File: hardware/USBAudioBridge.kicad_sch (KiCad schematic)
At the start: 0 parts

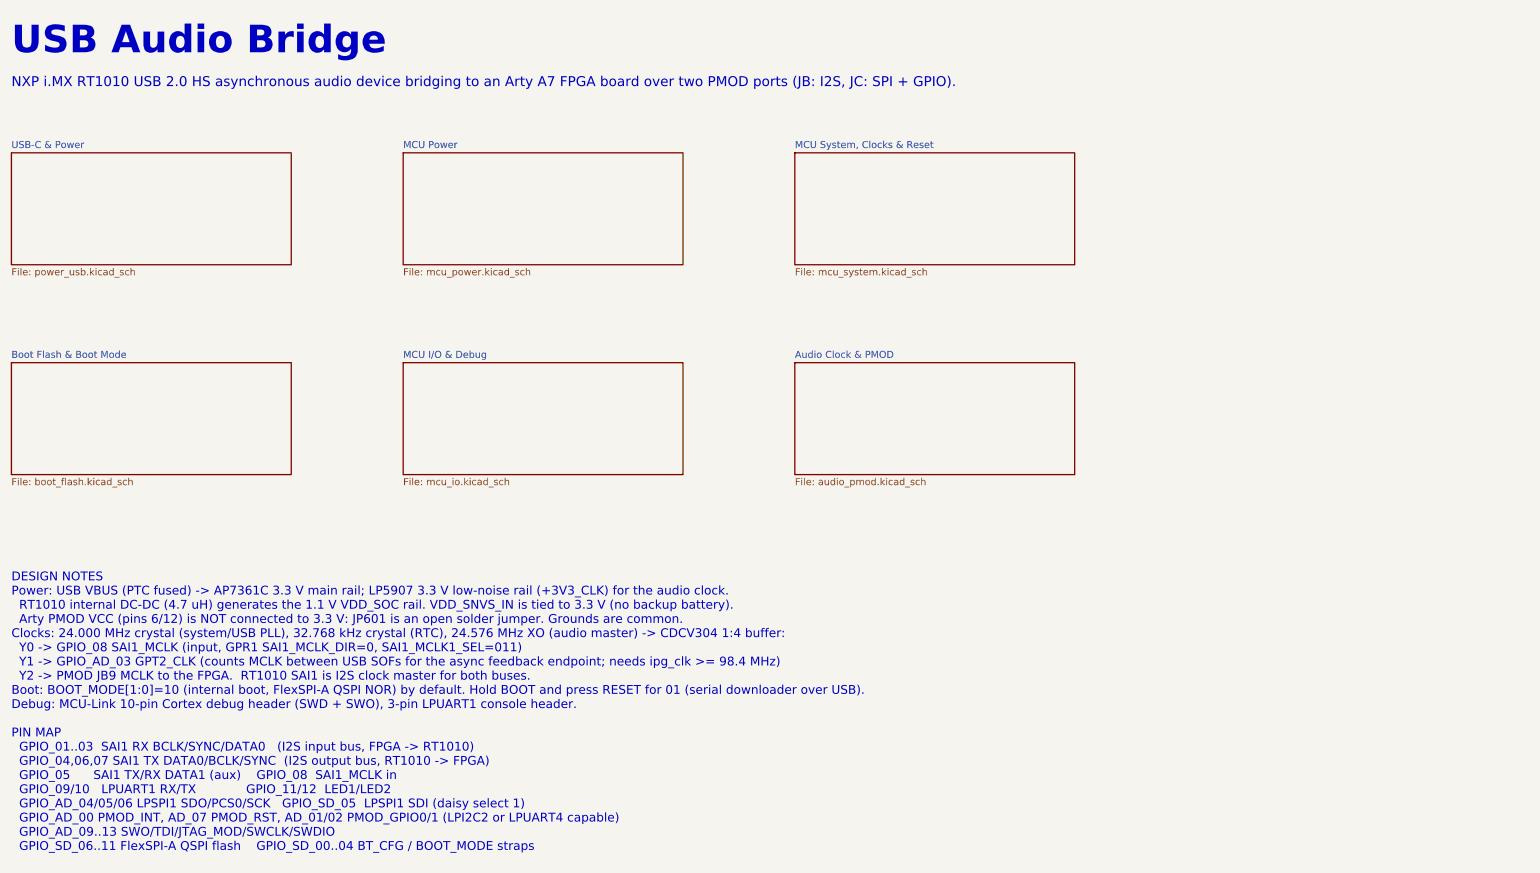
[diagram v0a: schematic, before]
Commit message: Post first draft design review complete
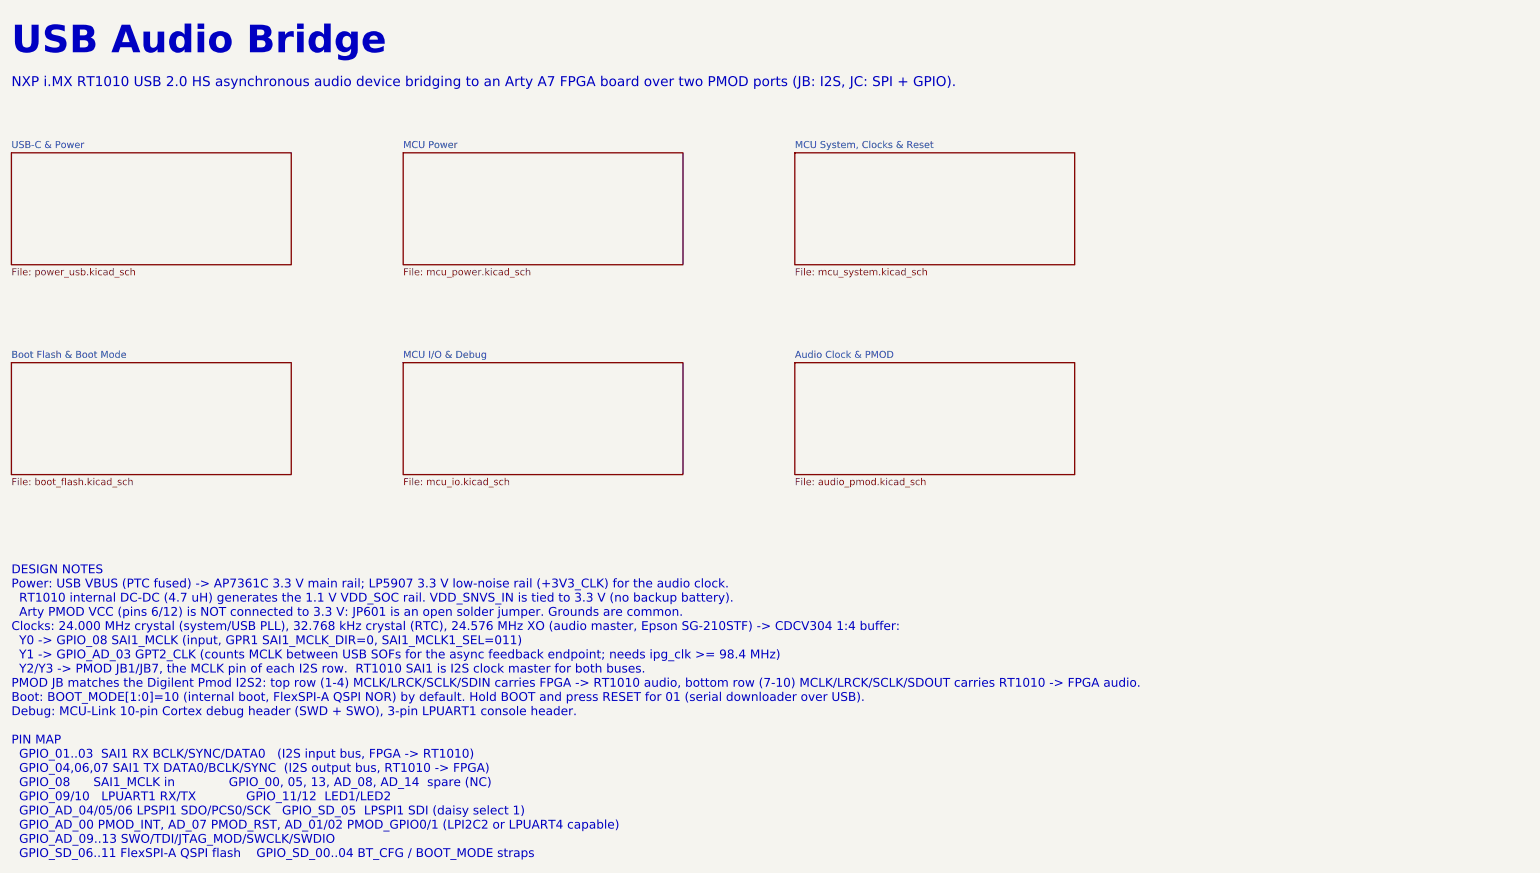
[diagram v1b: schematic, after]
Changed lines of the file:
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@@
 		)
 	)
-	(text "DESIGN NOTES\nPower: USB VBUS (PTC fused) -> AP7361C 3.3 V main rail; LP5907 3.3 V low-noise rail (+3V3_CLK) for the audio clock.\n  RT1010 internal DC-DC (4.7 uH) generates the 1.1 V VDD_SOC rail. VDD_SNVS_IN is tied to 3.3 V (no backup battery).\n  Arty PMOD VCC (pins 6/12) is NOT connected to 3.3 V: JP601 is an open solder jumper. Grounds are common.\nClocks: 24.000 MHz crystal (system/USB PLL), 32.768 kHz crystal (RTC), 24.576 MHz XO (audio master) -> CDCV304 1:4 buffer:\n  Y0 -> GPIO_08 SAI1_MCLK (input, GPR1 SAI1_MCLK_DIR=0, SAI1_MCLK1_SEL=011)\n  Y1 -> GPIO_AD_03 GPT2_CLK (counts MCLK between USB SOFs for the async feedback endpoint; needs ipg_clk >= 98.4 MHz)\n  Y2 -> PMOD JB9 MCLK to the FPGA.  RT1010 SAI1 is I2S clock master for both buses.\nBoot: BOOT_MODE[1:0]=10 (internal boot, FlexSPI-A QSPI NOR) by default. Hold BOOT and press RESET for 01 (serial downloader over USB).\nDebug: MCU-Link 10-pin Cortex debug header (SWD + SWO), 3-pin LPUART1 console header.\n\nPIN MAP\n  GPIO_01..03  SAI1 RX BCLK/SYNC/DATA0   (I2S input bus, FPGA -> RT1010)\n  GPIO_04,06,07 SAI1 TX DATA0/BCLK/SYNC  (I2S output bus, RT1010 -> FPGA)\n  GPIO_05      SAI1 TX/RX DATA1 (aux)    GPIO_08  SAI1_MCLK in\n  GPIO_09/10   LPUART1 RX/TX             GPIO_11/12  LED1/LED2\n  GPIO_AD_04/05/06 LPSPI1 SDO/PCS0/SCK   GPIO_SD_05  LPSPI1 SDI (daisy select 1)\n  GPIO_AD_00 PMOD_INT, AD_07 PMOD_RST, AD_01/02 PMOD_GPIO0/1 (LPI2C2 or LPUART4 capable)\n  GPIO_AD_09..13 SWO/TDI/JTAG_MOD/SWCLK/SWDIO\n  GPIO_SD_06..11 FlexSPI-A QSPI flash    GPIO_SD_00..04 BT_CFG / BOOT_MODE straps"
+	(text "DESIGN NOTES\nPower: USB VBUS (PTC fused) -> AP7361C 3.3 V main rail; LP5907 3.3 V low-noise rail (+3V3_CLK) for the audio clock.\n  RT1010 internal DC-DC (4.7 uH) generates the 1.1 V VDD_SOC rail. VDD_SNVS_IN is tied to 3.3 V (no backup battery).\n  Arty PMOD VCC (pins 6/12) is NOT connected to 3.3 V: JP601 is an open solder jumper. Grounds are common.\nClocks: 24.000 MHz crystal (system/USB PLL), 32.768 kHz crystal (RTC), 24.576 MHz XO (audio master, Epson SG-210STF) -> CDCV304 1:4 buffer:\n  Y0 -> GPIO_08 SAI1_MCLK (input, GPR1 SAI1_MCLK_DIR=0, SAI1_MCLK1_SEL=011)\n  Y1 -> GPIO_AD_03 GPT2_CLK (counts MCLK between USB SOFs for the async feedback endpoint; needs ipg_clk >= 98.4 MHz)\n  Y2/Y3 -> PMOD JB1/JB7, the MCLK pin of each I2S row.  RT1010 SAI1 is I2S clock master for both buses.\nPMOD JB matches the Digilent Pmod I2S2: top row (1-4) MCLK/LRCK/SCLK/SDIN carries FPGA -> RT1010 audio, bottom row (7-10) MCLK/LRCK/SCLK/SDOUT carries RT1010 -> FPGA audio.\nBoot: BOOT_MODE[1:0]=10 (internal boot, FlexSPI-A QSPI NOR) by default. Hold BOOT and press RESET for 01 (serial downloader over USB).\nDebug: MCU-Link 10-pin Cortex debug header (SWD + SWO), 3-pin LPUART1 console header.\n\nPIN MAP\n  GPIO_01..03  SAI1 RX BCLK/SYNC/DATA0   (I2S input bus, FPGA -> RT1010)\n  GPIO_04,06,07 SAI1 TX DATA0/BCLK/SYNC  (I2S output bus, RT1010 -> FPGA)\n  GPIO_08      SAI1_MCLK in              GPIO_00, 05, 13, AD_08, AD_14  spare (NC)\n  GPIO_09/10   LPUART1 RX/TX             GPIO_11/12  LED1/LED2\n  GPIO_AD_04/05/06 LPSPI1 SDO/PCS0/SCK   GPIO_SD_05  LPSPI1 SDI (daisy select 1)\n  GPIO_AD_00 PMOD_INT, AD_07 PMOD_RST, AD_01/02 PMOD_GPIO0/1 (LPI2C2 or LPUART4 capable)\n  GPIO_AD_09..13 SWO/TDI/JTAG_MOD/SWCLK/SWDIO\n  GPIO_SD_06..11 FlexSPI-A QSPI flash    GPIO_SD_00..04 BT_CFG / BOOT_MODE straps"
 		(exclude_from_sim no)
 		(at 30.48 152.4 0)
